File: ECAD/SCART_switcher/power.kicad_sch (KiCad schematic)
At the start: 38 parts, among them SW1 SW_Push_DPDT, U12 L7805, U13 L7809

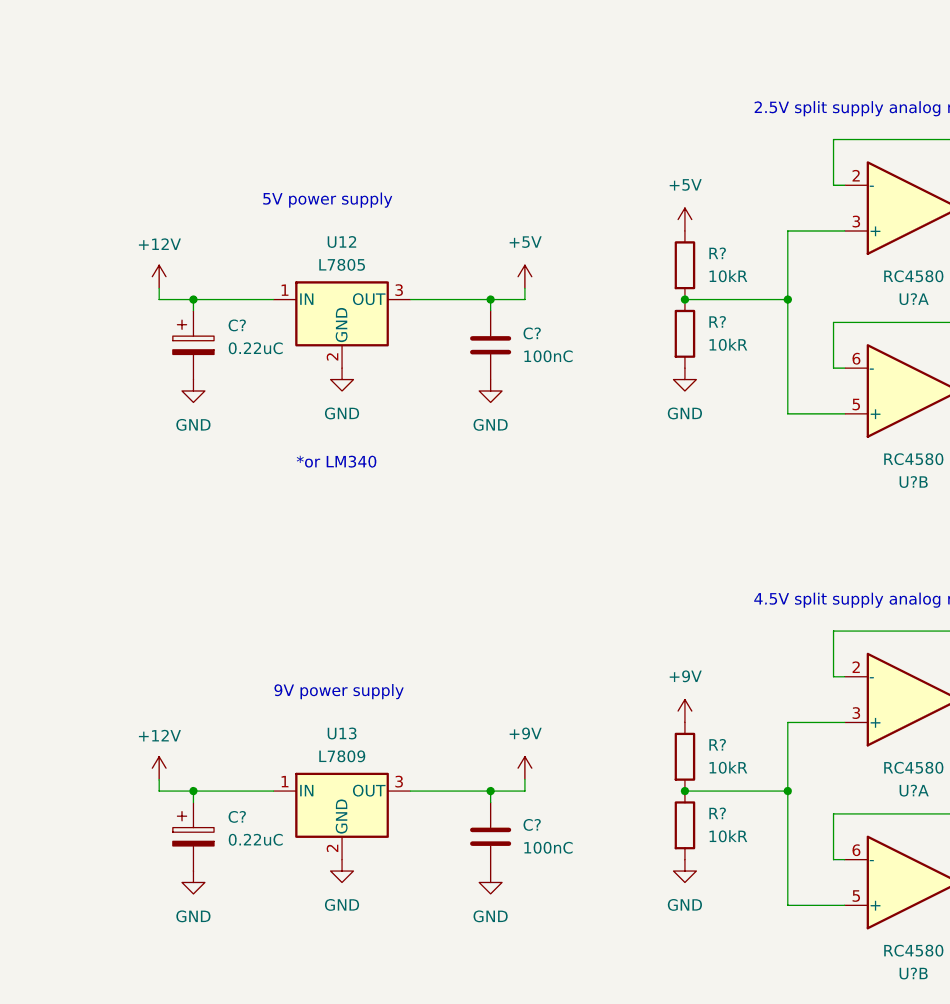
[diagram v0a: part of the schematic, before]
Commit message: progressed ecad
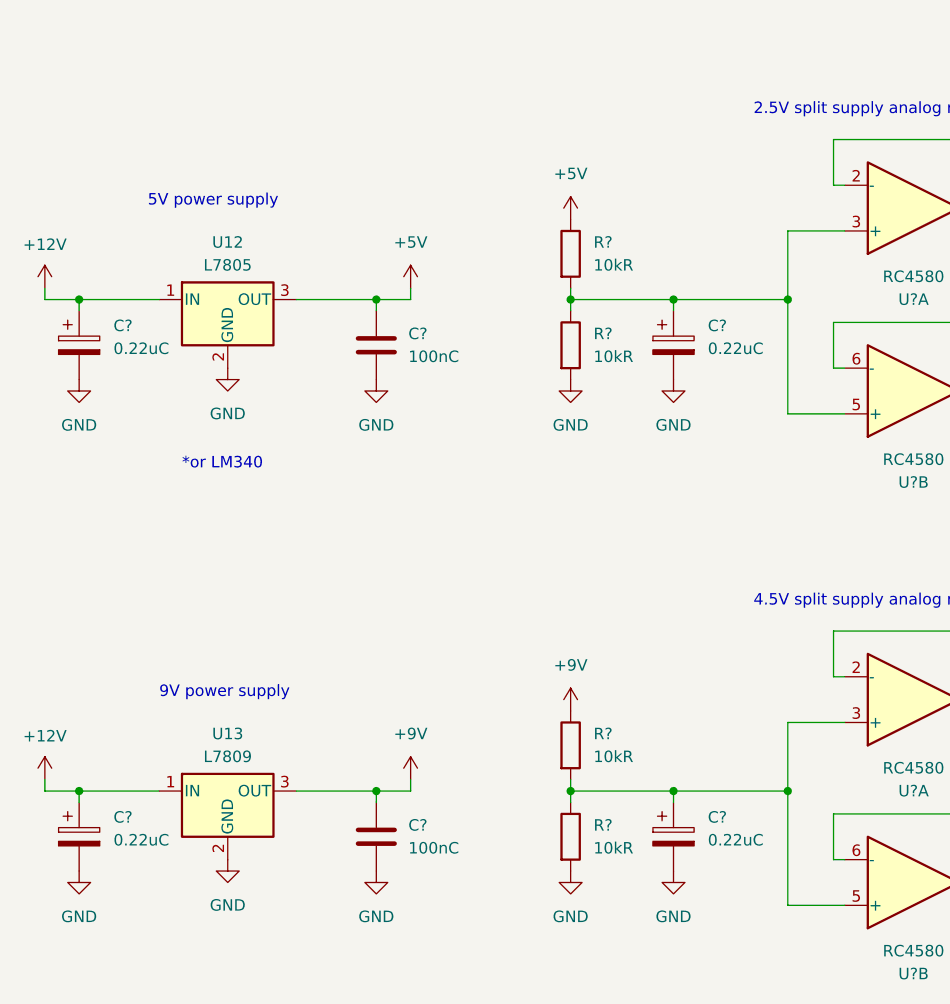
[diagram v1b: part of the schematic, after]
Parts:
- added C? (x2): 0.22uC, Capacitor_Tantalum_SMD:CP_EIA-3216-18_Kemet-A_Pad1.58x1.35mm_HandSolder, symbol Device:C_Polarized
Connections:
- net GND: now also C?.2, C?.2
- net at R?.1, R?.2, U?.3 (+)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: now also C?.1 (x2)
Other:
- moved on the sheet: C?, R?, U12, U13
